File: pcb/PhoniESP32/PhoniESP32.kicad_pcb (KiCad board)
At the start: 4 copper layers, 69 parts, among them J1 Connector, USB-TYPE-C-16P, J2 Conn_Battery, J3 Conn_Buttons, J4 Conn_01x08_Pin, J5 Screw_Terminal_01x02, SW1 SK12D07VG5, U1 TPS631000DRLR, U2 MAX98357AETE+T, U3 ESP32-C6-MINI-1-N4, U4 SPH0645LM4H-1-8_C19272537, U5 BQ24073RGTR

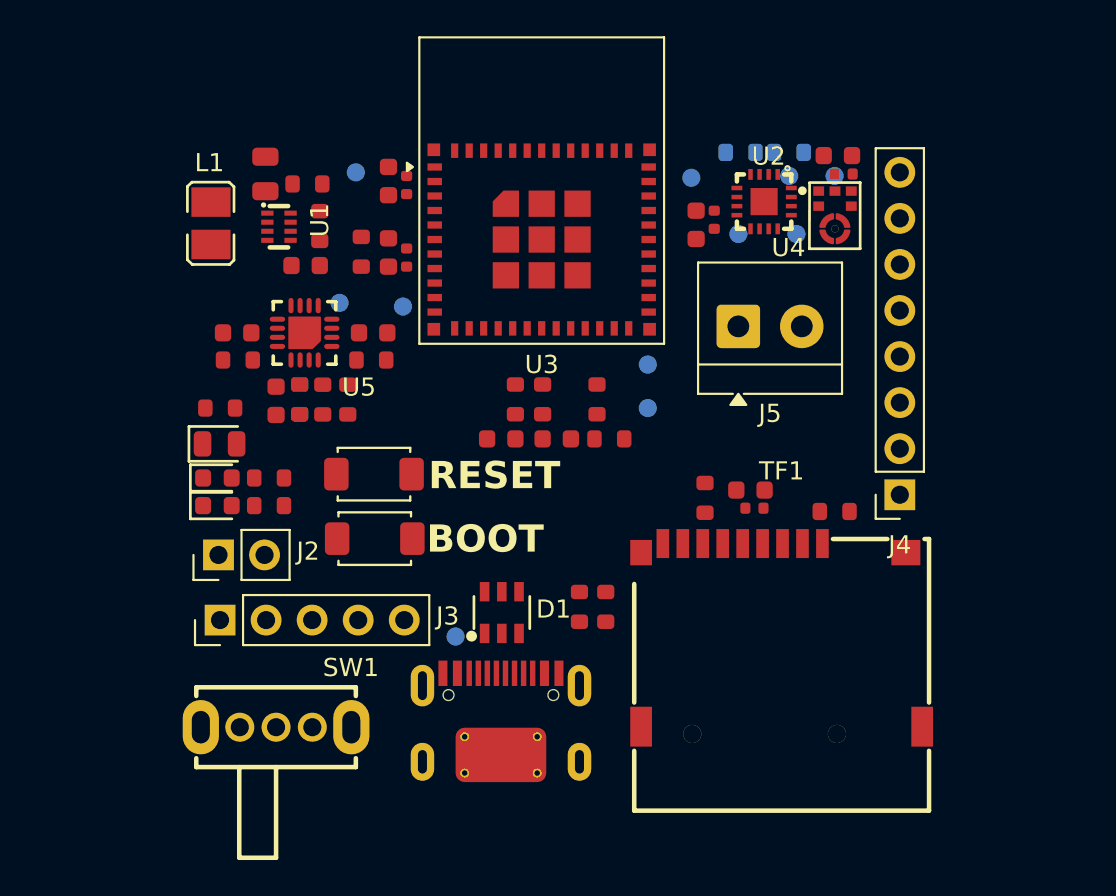
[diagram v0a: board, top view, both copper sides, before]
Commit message: feat(pcb): initial traces
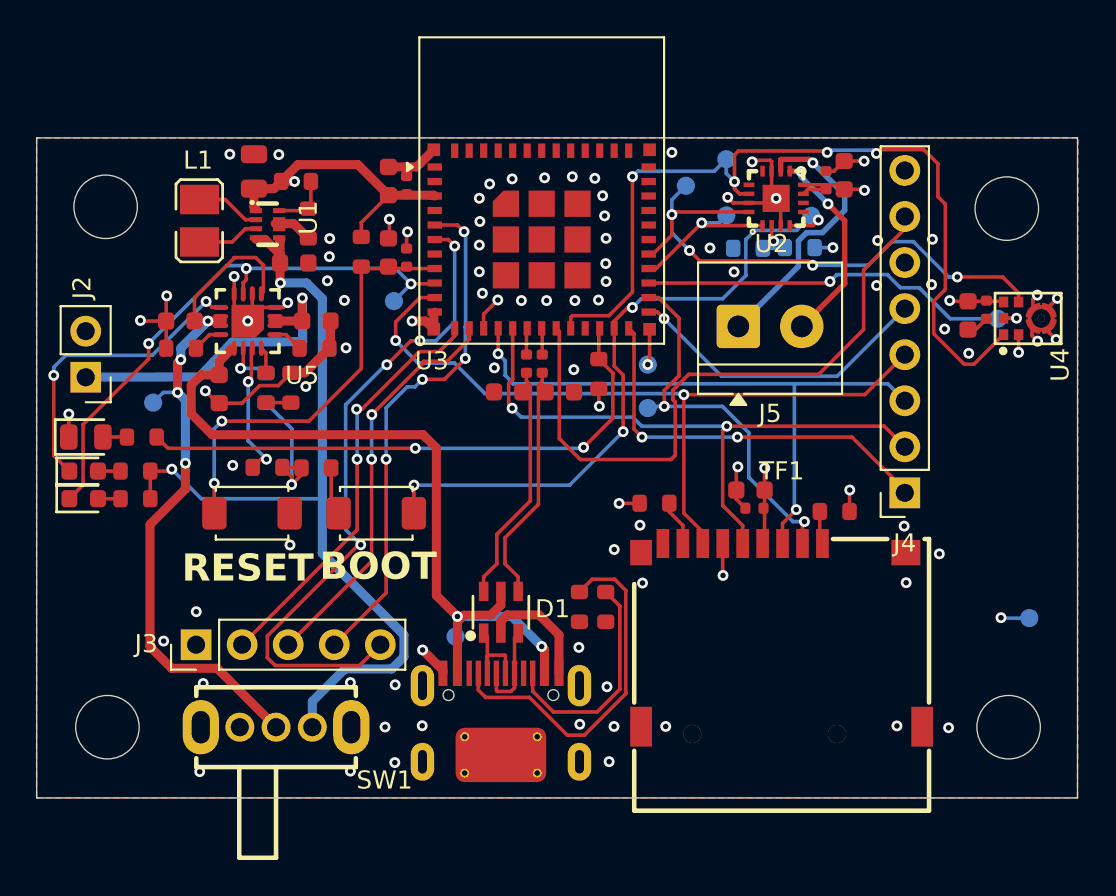
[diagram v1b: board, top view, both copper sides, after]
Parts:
- added REF**: MountingHole_3.5mm, MountingHole:MountingHole_3.5mm, F.Cu at (125.0, 118.9)
- added REF**: MountingHole_3.5mm, MountingHole:MountingHole_3.5mm, F.Cu at (174.6, 90.3)
- added REF**: MountingHole_3.5mm, MountingHole:MountingHole_3.5mm, F.Cu at (124.9, 90.2)
- added REF**: MountingHole_3.5mm, MountingHole:MountingHole_3.5mm, F.Cu at (174.7, 118.9)
- R10, R11: footprint PCM_JLCPCB:R_0603 -> PCM_JLCPCB:R_0402
- moved TP4 44.5 mm to (175.8, 112.9)
- moved R13 25.8 mm to (126.9, 102.9)
- moved J2 12.2 mm to (123.8, 99.6), turned to 180 degrees
- moved U4 12.0 mm to (175.7, 96.3), turned to 0 degrees
- moved TP8 12.0 mm to (174.1, 96.4), turned to -90 degrees
- moved TP5 11.7 mm to (127.5, 101.0)
- moved C15 11.4 mm to (172.5, 96.2), turned to -90 degrees
- moved C14 10.9 mm to (173.5, 95.9), turned to -90 degrees
- moved C12 8.61 mm to (165.6, 88.5), turned to 90 degrees
- moved D2 7.38 mm to (123.7, 106.3)
- moved D3 7.38 mm to (123.7, 104.8)
- moved D4 7.38 mm to (123.8, 102.9)
- moved R6 7.38 mm to (126.5, 104.8)
- moved R7 7.38 mm to (126.5, 106.3)
- moved S1 7.06 mm to (133.0, 107.1)
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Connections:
- net Net-(D1-Pad1) renamed /Power/D-
- net Net-(D1-Pad3) renamed /Power/D+
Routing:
- net GND: track 0.00 -> 76.6 mm, vias 0 -> 88
- net +5V: track 0.00 -> 48.1 mm, vias 0 -> 2
- net /I2S_WS: track 0.00 -> 48.0 mm, vias 0 -> 4
- net VBUS: track 0.00 -> 43.9 mm, vias 0 -> 2
- net /SPI_MISO: track 0.00 -> 42.6 mm, vias 0 -> 2
- net Net-(U5-EN2): track 0.00 -> 39.4 mm, vias 0 -> 4
- net /AUDIO_EN: track 0.00 -> 37.2 mm, vias 0 -> 4
- net /BTN_VOL_UP: track 0.00 -> 36.7 mm, vias 0 -> 4
- net /RFID_EN: track 0.00 -> 35.8 mm
- net +3.3V: track 0.00 -> 35.0 mm, vias 0 -> 10
- net /SPI_MOSI: track 0.00 -> 34.6 mm, vias 0 -> 2
- net /SPI_SCK: track 0.00 -> 34.1 mm, vias 0 -> 2
- net /I2S_BCLK: track 0.00 -> 32.1 mm, vias 0 -> 4
- net Net-(U3-IO8): track 0.00 -> 31.4 mm, vias 0 -> 2
- net /CHARGER: track 0.00 -> 31.2 mm, vias 0 -> 3
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- added copper zone on In2.Cu, net +3.3V
- added copper zone on B.Cu, net GND
- added copper zone on F.Cu, net GND
- added copper zone on In1.Cu, net GND
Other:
- board outline added: 57.4 x 36.4 mm
